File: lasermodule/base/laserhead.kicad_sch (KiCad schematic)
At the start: 39 parts, among them J3 Conn_01x02, J4 Conn_01x03, J5 Conn_01x02, J6 jumper wire 2 pin, U1 DIGIPOT_50K, U11 LM7808_TO220, U2 U_IC-HKB, U3 STSPIN230, U4 MIC920, U5 MIC920, U6 DRV5033FAxDBZ, U7 DRV5033FAxDBZ, U8 DRV5033FAxDBZ

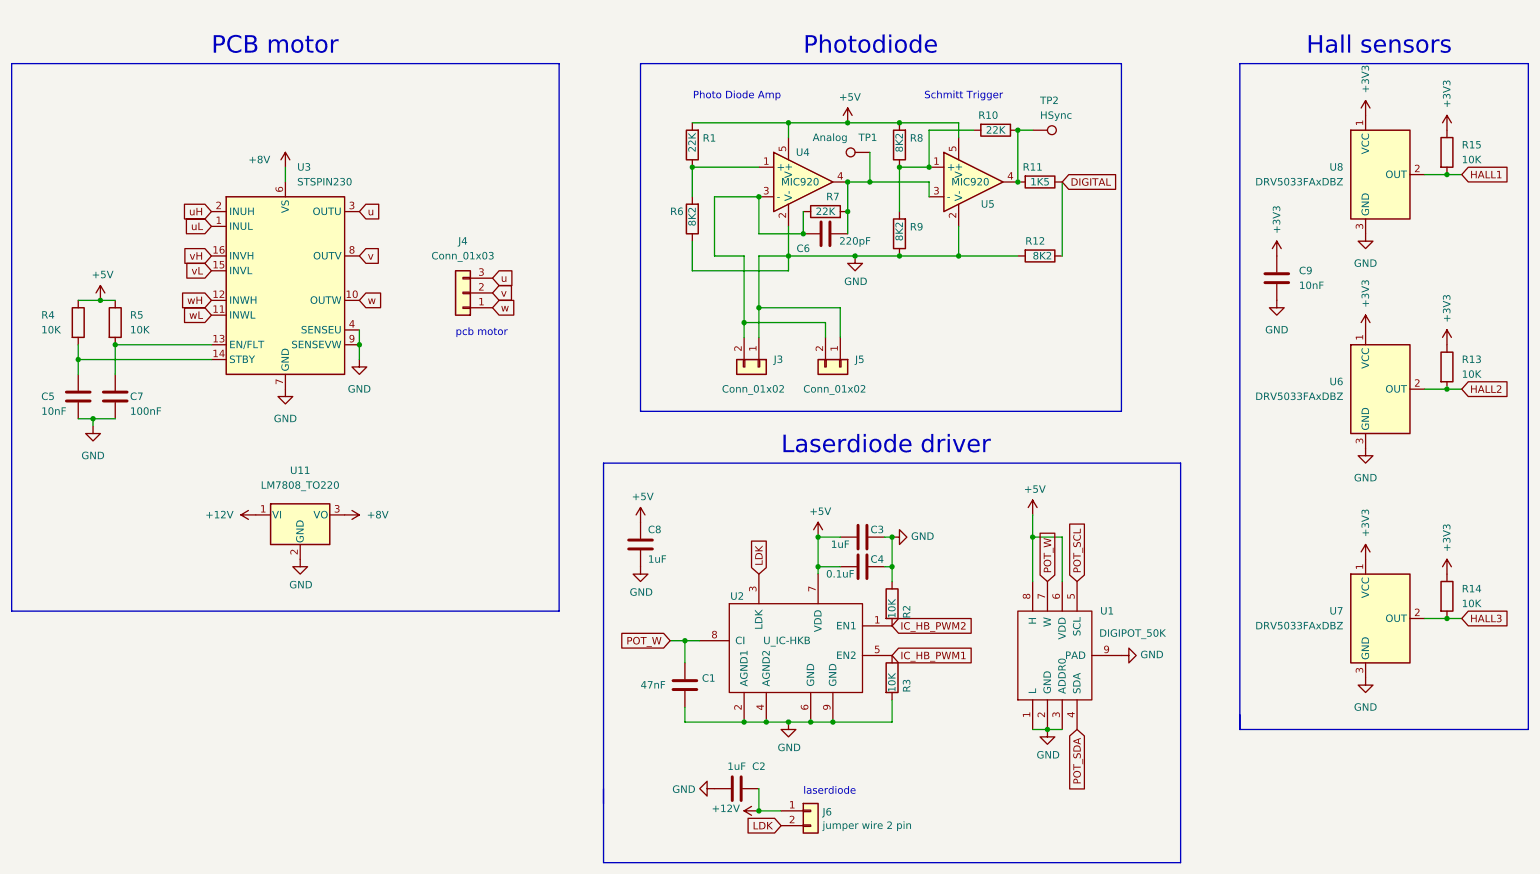
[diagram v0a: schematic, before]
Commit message: board almost fully synced close for release
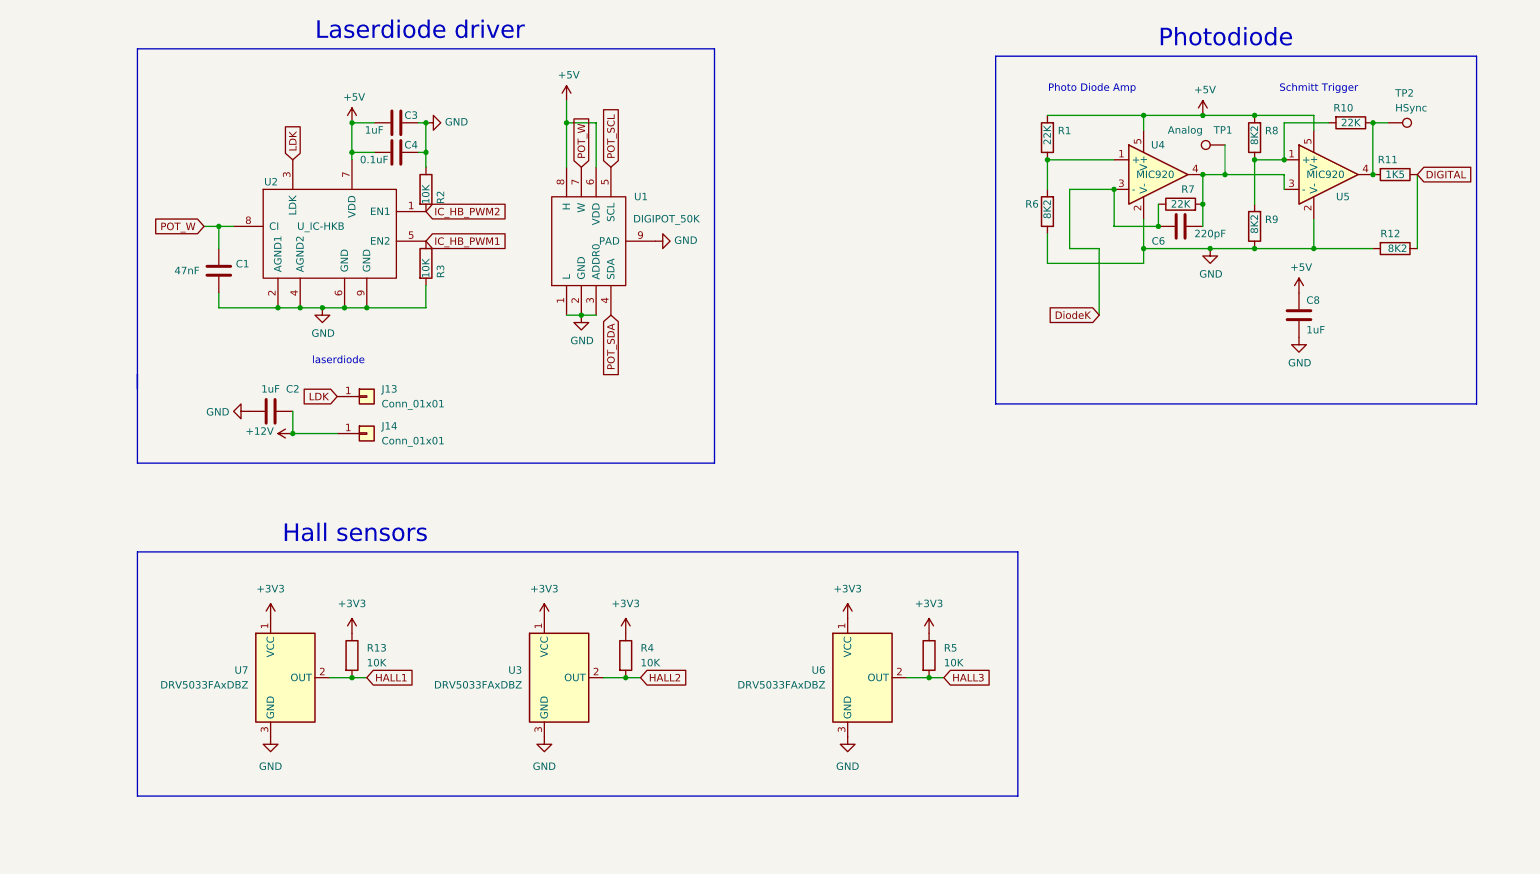
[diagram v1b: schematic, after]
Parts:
- removed C5, C9: 10nF, Capacitor_SMD:C_0805_2012Metric_Pad1.18x1.45mm_HandSolder, symbol Device:C
- removed C7: 100nF, Capacitor_SMD:C_0805_2012Metric_Pad1.18x1.45mm_HandSolder, symbol Device:C
- removed J3, J5: Conn_01x02, sockets_scanhead:PinHeader_1x02_P2.54mm_Vertical, symbol Connector_Generic:Conn_01x02
- removed J4: Conn_01x03, sockets_scanhead:pcbmotor_smd, symbol Connector_Generic:Conn_01x03
- removed J6: jumper wire 2 pin, Connector_Molex:Molex_KK-254_AE-6410-02A_1x02_P2.54mm_Vertical, symbol Connector_Generic:Conn_01x02
- removed R14, R15: 10K, Resistor_SMD:R_0805_2012Metric_Pad1.20x1.40mm_HandSolder, symbol Device:R
- removed U11: LM7808_TO220, Package_TO_SOT_THT:TO-220-3_Vertical, symbol Regulator_Linear:LM7805_TO220
- removed U3: STSPIN230, sockets_scanhead:VQFN-16-1EP_3x3mm_P0.5mm_EP1.8x1.8mm, symbol Driver_Motor:STSPIN230
- removed U8: DRV5033FAxDBZ, Package_TO_SOT_SMD:SOT-23, symbol Sensor_Magnetic:DRV5033FAxDBZ
- added J13, J14: Conn_01x01, sockets_scanhead:throughholeplate, symbol Connector_Generic:Conn_01x01
- added U3: DRV5033FAxDBZ, Package_TO_SOT_SMD:SOT-23, symbol Sensor_Magnetic:DRV5033FAxDBZ
- U1: Mouser (none) -> 700-MAX5395MATA+T; Price (none) -> 2,36; Producer (none) -> MAX5395
- U2: Price (none) -> 2.9; Producer (none) -> iC-HK SO8-TP or ic-hkbmsop8
- U4, U5: Farnell (none) -> 2920854; Mouser (none) -> 998-MIC920YC5TR; Price (none) -> 0,44
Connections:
- net +12V: now also J14.1 (Pin_1)
- net +3V3: now also R4.1, R5.1, U3.1 (VCC)
- net +5V: no longer R4.1, R5.1
- net GND: now also U3.3 (GND)
- net HALL1: now also R13.2, U7.2 (OUT)
- net HALL2: now also R4.2, U3.2 (OUT); no longer R13.2, U6.2 (OUT)
- net HALL3: now also R5.2, U6.2 (OUT); no longer U7.2 (OUT)
- net LDK: now also J13.1 (Pin_1)
- net DiodeK: now reaches C6.2, R7.1, U4.3 (-)
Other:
- note removed: "PCB motor"
- note removed: "pcb motor"
- moved on the sheet: C1, C2, C3, C4, C6, C8, R1, R10, R11, R12, R2, R3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
